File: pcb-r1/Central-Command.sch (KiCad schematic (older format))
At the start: 18 parts, among them P101 CONN_01X10, P102 CONN_01X10, P103 CONN_01X04, P104 CONN_01X02, P105 CONN_01X04, P106 CONN_01X02, U101 STM32F030C8, Y101 Crystal

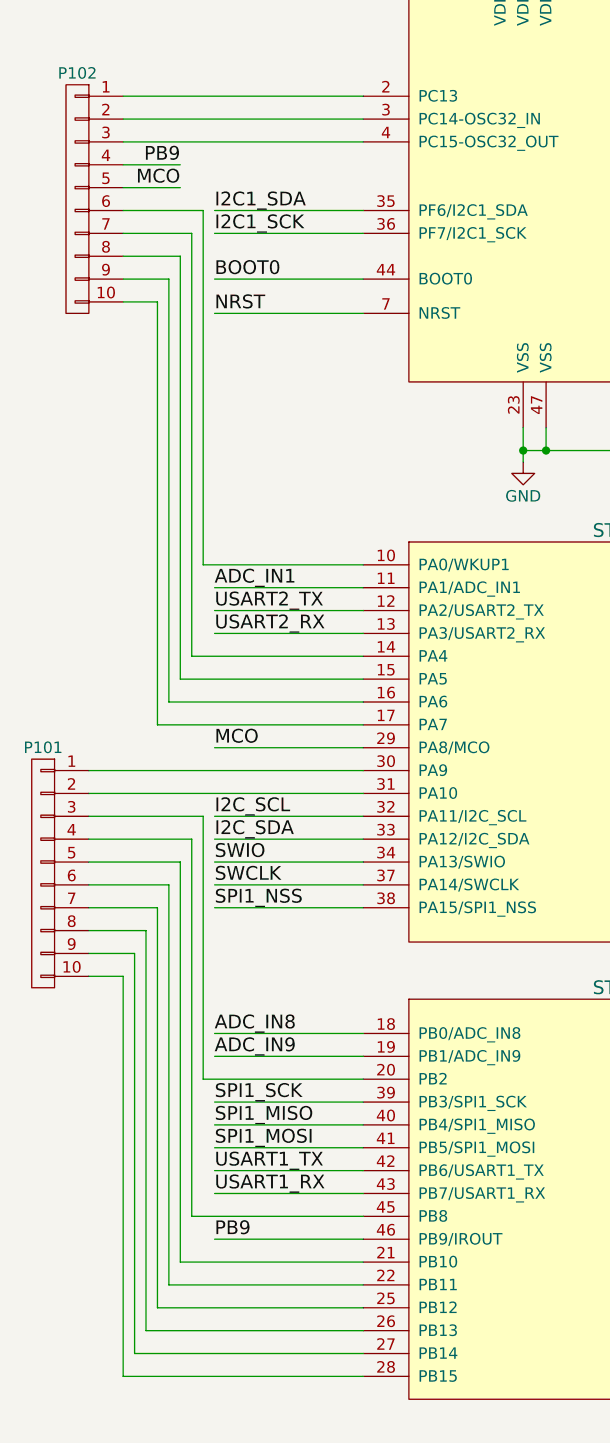
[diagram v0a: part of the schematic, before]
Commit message: Completed the layout. Saving before sending off to Fab.
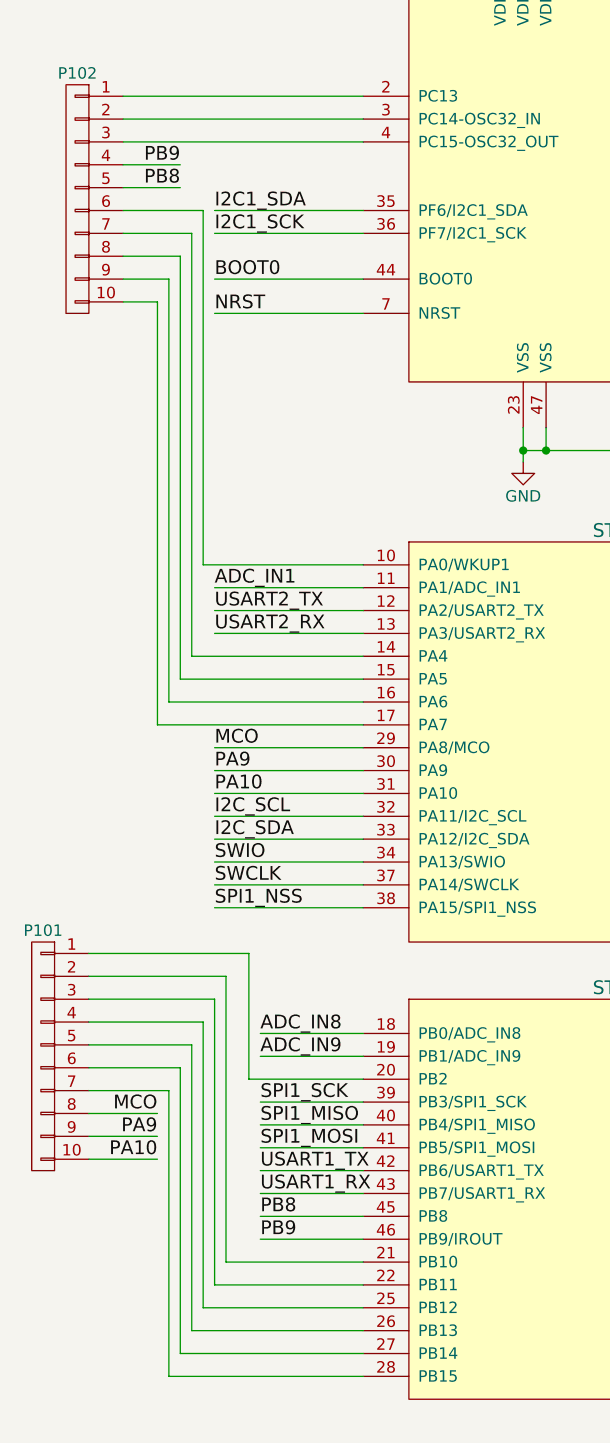
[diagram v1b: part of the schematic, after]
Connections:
- net MCO: now also P101.8 (P8); no longer P102.5 (P5)
- net at P101.1 (P1): now also U101.20 (PB2); no longer U101.30 (PA9)
- net at P101.2 (P2): now also U101.21 (PB10); no longer U101.31 (PA10)
- net at P101.3 (P3): now also U101.22 (PB11); no longer U101.20 (PB2)
- net at P101.5 (P5): now also U101.26 (PB13); no longer U101.21 (PB10)
- net at P101.6 (P6): now also U101.27 (PB14); no longer U101.22 (PB11)
- net at U101.25 (PB12): now also P101.4 (P4); no longer P101.7 (P7)
- net PA9: now reaches P101.9 (P9)
- net PA9: now also U101.30 (PA9); no longer U101.27 (PB14)
- net at U101.28 (PB15): now also P101.7 (P7); no longer P101.10 (P10)
- net PB8: now reaches U101.45 (PB8)
- net PB8: now also P102.5 (P5); no longer P101.4 (P4)
- new net PA10: P101.10 (P10), U101.31 (PA10)
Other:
- moved on the sheet: P101
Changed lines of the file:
@@
 L CONN_01X10 P101
 U 1 1 56677880
-P 700 5100
-F 0 "P101" H 700 5650 50  0000 C CNN
-F 1 "CONN_01X10" V 800 5100 50  0001 C CNN
-F 2 "Pin_Headers:Pin_Header_Straight_1x10" H 700 5100 60  0001 C CNN
-F 3 "" H 700 5100 60  0000 C CNN
-	1    700  5100
+P 700 5900
+F 0 "P101" H 700 6450 50  0000 C CNN
+F 1 "CONN_01X10" V 800 5900 50  0001 C CNN
+F 2 "Pin_Headers:Pin_Header_Straight_1x10" H 700 5900 60  0001 C CNN
+F 3 "" H 700 5900 60  0000 C CNN
+	1    700  5900
 	-1   0    0    -1
 $EndComp
@@
 Text Label 1450 5250 0    60   ~ 0
 SPI1_NSS
-Text Label 1450 5800 0    60   ~ 0
+Text Label 1650 5800 0    60   ~ 0
 ADC_IN8
-Text Label 1450 5900 0    60   ~ 0
+Text Label 1650 5900 0    60   ~ 0
 ADC_IN9
-Text Label 1450 6100 0    60   ~ 0
+Text Label 1650 6100 0    60   ~ 0
 SPI1_SCK
-Text Label 1450 6200 0    60   ~ 0
+Text Label 1650 6200 0    60   ~ 0
 SPI1_MISO
-Text Label 1450 6300 0    60   ~ 0
+Text Label 1650 6300 0    60   ~ 0
 SPI1_MOSI
-Text Label 1450 6400 0    60   ~ 0
+Text Label 1650 6400 0    60   ~ 0
 USART1_TX
-Text Label 1450 6500 0    60   ~ 0
+Text Label 1650 6500 0    60   ~ 0
 USART1_RX
-Text Label 1450 6700 0    60   ~ 0
+Text Label 1650 6700 0    60   ~ 0
 PB9
 Text Label 1450 2200 0    60   ~ 0
@@
 Text Label 1300 2000 2    60   ~ 0
 PB9
-Text Label 1300 2100 2    60   ~ 0
+Text Label 1200 6150 2    60   ~ 0
 MCO
 Text Label 1450 3850 0    60   ~ 0
@@
 Text Label 7200 900  0    60   ~ 0
 PWR
+Text Label 1450 4650 0    60   ~ 0
+PA9
+Text Label 1450 4750 0    60   ~ 0
+PA10
+Text Label 1200 6250 2    60   ~ 0
+PA9
+Text Label 1200 6350 2    60   ~ 0
+PA10
+Text Label 1650 6600 0    60   ~ 0
+PB8
+Text Label 1300 2100 2    60   ~ 0
+PB8
 Wire Wire Line
 	2950 800  2900 800
@@
 	8550 4800 8100 4800
 Wire Wire Line
-	900  4650 2100 4650
-Wire Wire Line
-	900  4750 2100 4750
-Wire Wire Line
 	2100 4850 1450 4850
 Wire Wire Line
@@
 	2100 5250 1450 5250
 Wire Wire Line
-	900  4850 1400 4850
-Wire Wire Line
-	1400 4850 1400 6000
-Wire Wire Line
-	1400 6000 2100 6000
-Wire Wire Line
-	900  4950 1350 4950
-Wire Wire Line
-	1350 4950 1350 6600
-Wire Wire Line
-	1350 6600 2100 6600
-Wire Wire Line
-	900  5050 1300 5050
-Wire Wire Line
-	1300 5050 1300 6800
-Wire Wire Line
-	1300 6800 2100 6800
-Wire Wire Line
-	900  5150 1250 5150
-Wire Wire Line
-	1250 5150 1250 6900
-Wire Wire Line
-	1250 6900 2100 6900
-Wire Wire Line
-	900  5250 1200 5250
-Wire Wire Line
-	1200 5250 1200 7000
-Wire Wire Line
-	1200 7000 2100 7000
-Wire Wire Line
-	900  5350 1150 5350
-Wire Wire Line
-	1150 5350 1150 7100
-Wire Wire Line
-	1150 7100 2100 7100
-Wire Wire Line
-	900  5450 1100 5450
-Wire Wire Line
-	1100 5450 1100 7200
-Wire Wire Line
-	1100 7200 2100 7200
-Wire Wire Line
-	900  5550 1050 5550
-Wire Wire Line
-	1050 5550 1050 7300
-Wire Wire Line
-	1050 7300 2100 7300
-Wire Wire Line
-	2100 5800 1450 5800
-Wire Wire Line
-	2100 6100 1450 6100
-Wire Wire Line
-	2100 6200 1450 6200
-Wire Wire Line
-	2100 6300 1450 6300
-Wire Wire Line
-	2100 6500 1450 6500
-Wire Wire Line
-	2100 6400 1450 6400
-Wire Wire Line
-	2100 6700 1450 6700
-Wire Wire Line
-	2100 5900 1450 5900
+	1600 6000 2100 6000
+Wire Wire Line
+	900  5550 1500 5550
+Wire Wire Line
+	1500 5550 1500 6800
+Wire Wire Line
+	1500 6800 2100 6800
+Wire Wire Line
+	900  5650 1450 5650
+Wire Wire Line
+	1450 5650 1450 6900
+Wire Wire Line
+	1450 6900 2100 6900
+Wire Wire Line
+	900  5750 1400 5750
+Wire Wire Line
+	1400 5750 1400 7000
+Wire Wire Line
+	1400 7000 2100 7000
+Wire Wire Line
+	900  5850 1350 5850
+Wire Wire Line
+	1350 5850 1350 7100
+Wire Wire Line
+	1350 7100 2100 7100
+Wire Wire Line
+	900  5950 1300 5950
+Wire Wire Line
+	1300 5950 1300 7200
+Wire Wire Line
+	1300 7200 2100 7200
+Wire Wire Line
+	900  6050 1250 6050
+Wire Wire Line
+	1250 6050 1250 7300
+Wire Wire Line
+	1250 7300 2100 7300
+Wire Wire Line
+	2100 5800 1650 5800
+Wire Wire Line
+	2100 6100 1650 6100
+Wire Wire Line
+	2100 6200 1650 6200
+Wire Wire Line
+	2100 6300 1650 6300
+Wire Wire Line
+	2100 6500 1650 6500
+Wire Wire Line
+	2100 6400 1650 6400
+Wire Wire Line
+	2100 6700 1650 6700
+Wire Wire Line
+	2100 5900 1650 5900
 Wire Wire Line
 	2100 2650 1450 2650
@@
 	8100 1750 8100 1600
 Connection ~ 8100 1600
+Wire Wire Line
+	2100 4650 1450 4650
+Wire Wire Line
+	2100 4750 1450 4750
+Wire Wire Line
+	900  6150 1200 6150
+Wire Wire Line
+	900  6250 1200 6250
+Wire Wire Line
+	2100 6600 1650 6600
+Wire Wire Line
+	900  5450 1600 5450
+Wire Wire Line
+	900  6350 1200 6350
+Wire Wire Line
+	1600 5450 1600 6000
 $EndSCHEMATC
